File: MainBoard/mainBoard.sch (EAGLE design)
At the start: 77 parts, among them IC1 74HC238, IC2 74HC238, IC3 74HC151D, J1 22-05-7038-03, J2 22-05-7038-03, J3 22-05-7038-03, J4 22-05-7038-03, J5 22-05-7038-03, J6 22-05-7038-03, J7 22-05-7038-03, J8 22-05-7038-03, Q1 BC847ASMD, Q10 BC847ASMD, Q2 BC847ASMD, Q5 BC847ASMD, Q6 BC847ASMD, Q9 BC847ASMD, X1 PWR12, X2 MSTBA2, X3 MSTBA2, X4 MSTBA2, X5 MSTBA2, X6 MSTBA2, X7 MSTBA2

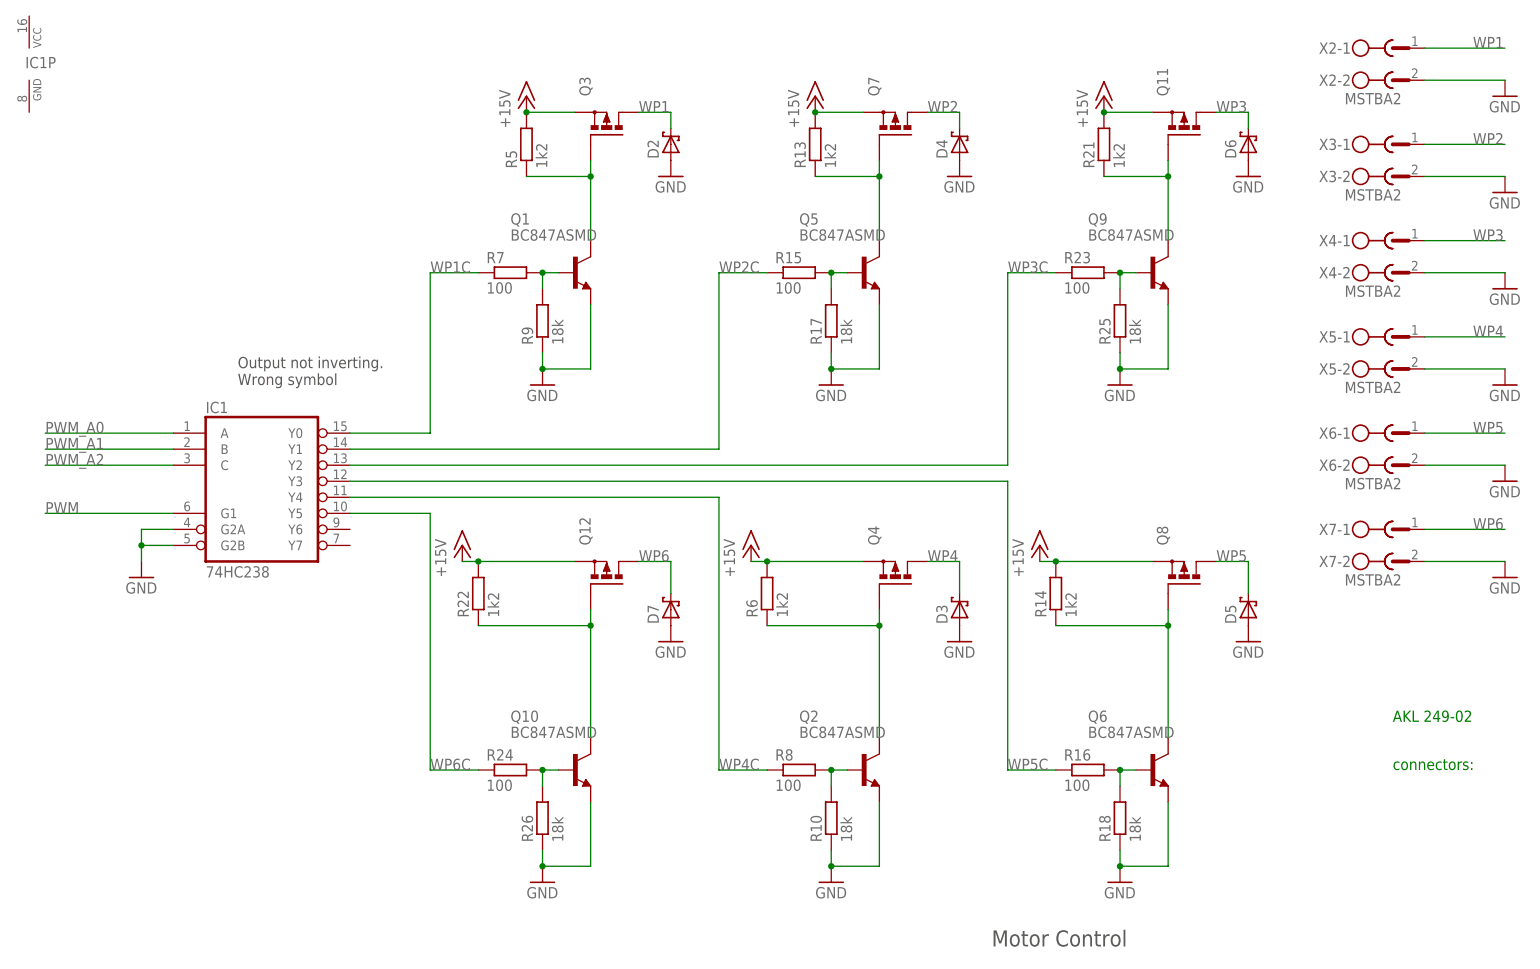
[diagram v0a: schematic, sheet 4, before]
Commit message: mainboard updates
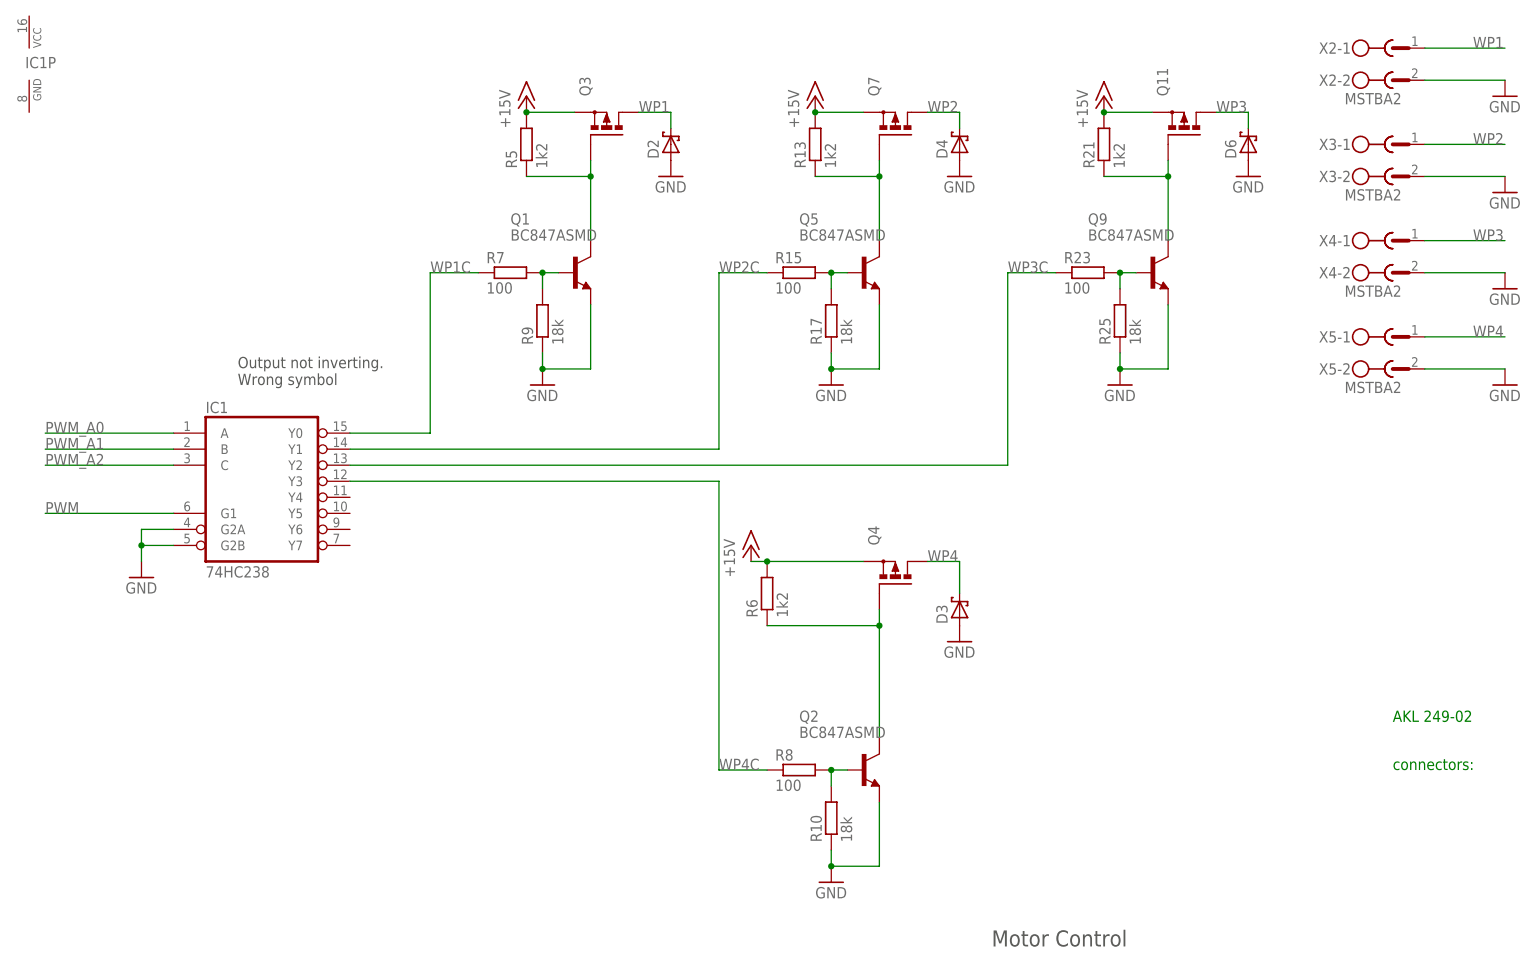
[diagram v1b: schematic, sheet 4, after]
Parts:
- removed D5, D7: (no value), diode:SCHOTTKY-DIODESMC
- removed Q10, Q6: BC847ASMD, transistor-npn:BC847ASMD
- removed Q12, Q8: (no value), transistor-power:P-MOSFET-SO8
- removed R14, R22: 1k2, rcl:R-EU_R0805
- removed R16, R24: 100, rcl:R-EU_R0805
- removed R18, R26: 18k, rcl:R-EU_R0805
- removed X6, X7: MSTBA2, con-phoenix-508:MSTBA2
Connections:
- removed net N$17: Q6.C, Q8.G, R14.1
- removed net N$18: Q6.B, R16.2, R18.2
- removed net N$21: Q10.C, Q12.G, R22.1
- removed net N$22: Q10.B, R24.2, R26.2
- removed net WP5: D5.C, Q8.D, X6-1.1
- removed net WP5C: IC1A.Y3, R16.1
- removed net WP6: D7.C, Q12.D, X7-1.1
- removed net WP6C: IC1A.Y5, R24.1
- net +15V: no longer Q12.S, Q8.S, R14.2, R22.2
- net GND: no longer D5.A, D7.A, Q10.E, Q6.E, R18.1, R26.1, X6-2.1, X7-2.1
- net WP4C: now also IC1A.Y3; no longer IC1A.Y4
